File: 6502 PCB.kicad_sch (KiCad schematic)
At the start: 23 parts, among them J1 power_source, SW1 RESET, SW2 SW_Push, SW3 SW_Push, SW4 SW_Push, SW5 SW_Push, SW6 SW_Push, U1 W65C02S, U2 28C256, U3 62256, U4 W65C22, U5 74HC00, X1 1MHz

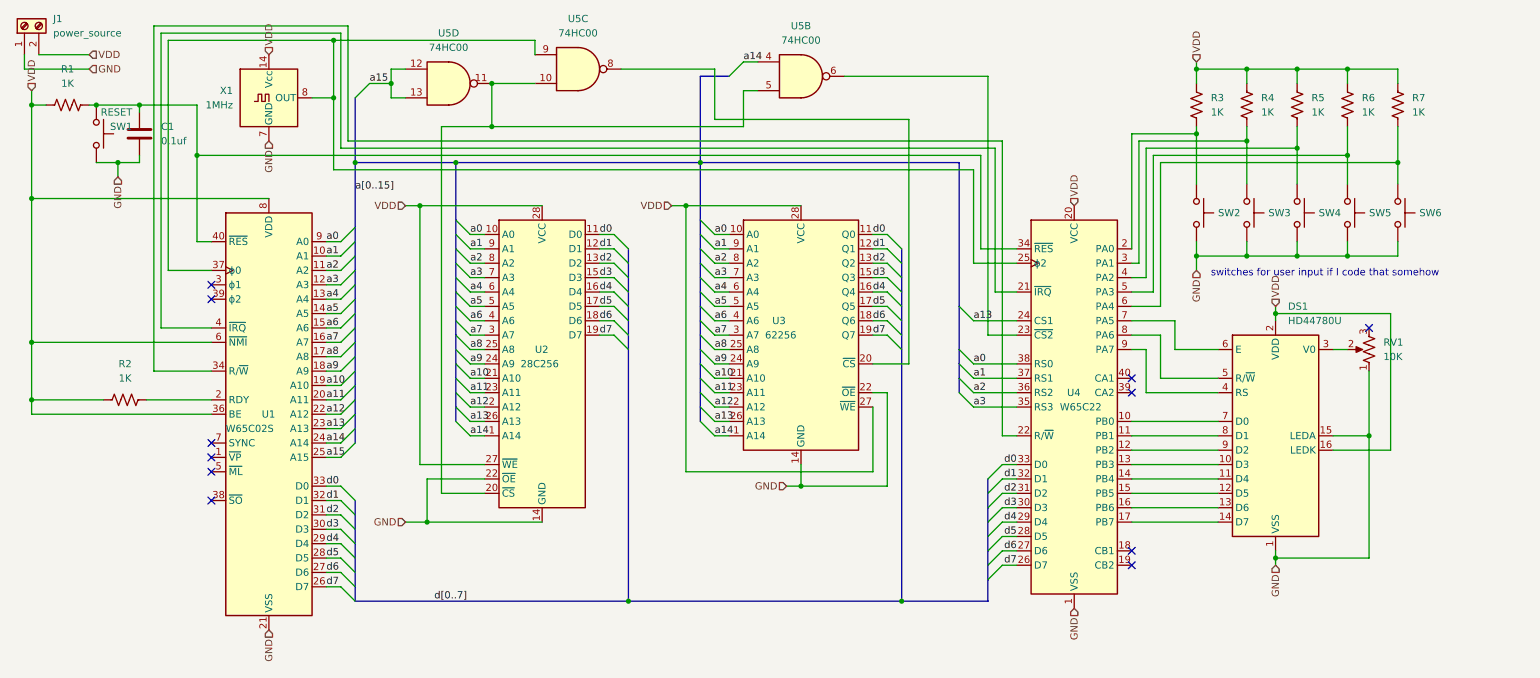
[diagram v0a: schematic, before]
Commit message: pretty much done
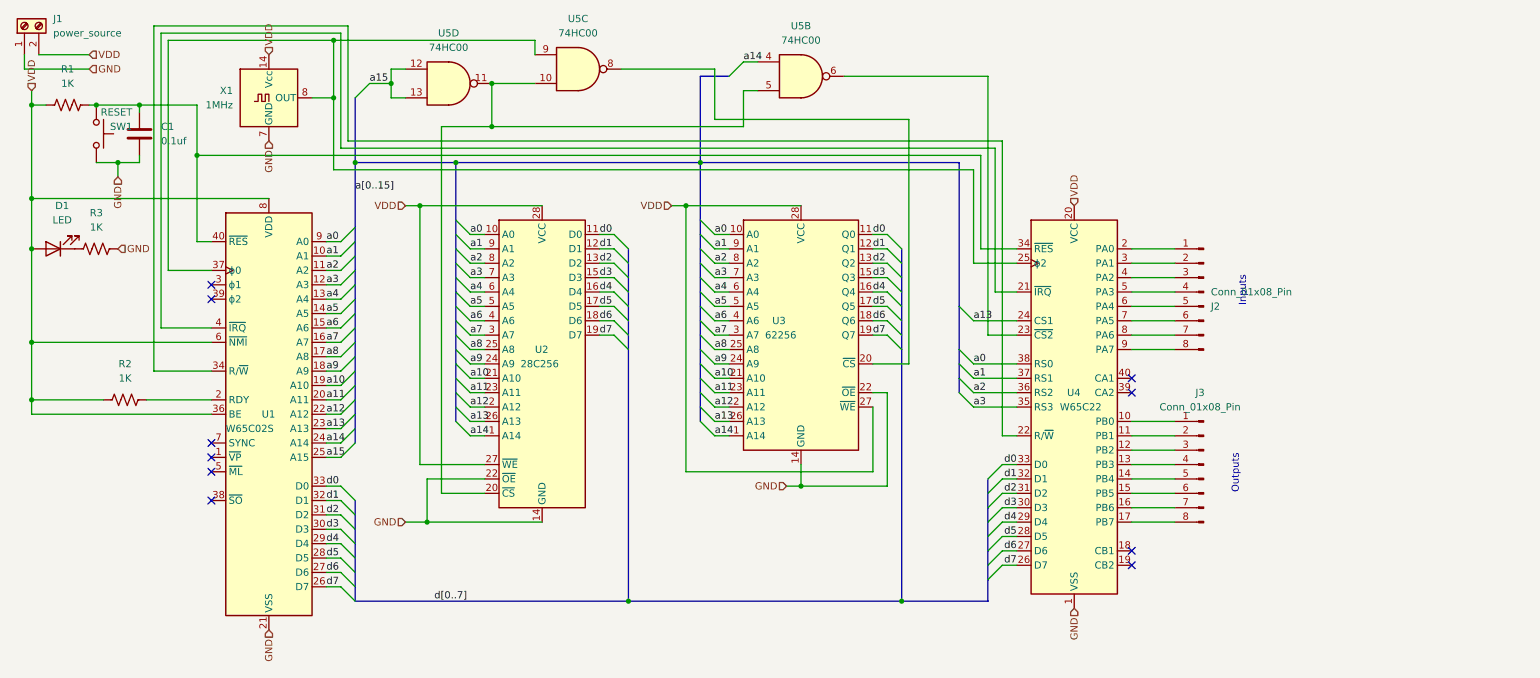
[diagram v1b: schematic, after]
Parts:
- removed DS1: HD44780U, Display:WC1602A, symbol HD44780U:HD44780U
- removed R4, R5, R6, R7: 1K, Resistor_SMD:R_0201_0603Metric_Pad0.64x0.40mm_HandSolder, symbol Device:R_US
- removed RV1: 10K, Potentiometer_SMD:Potentiometer_ACP_CA6-VSMD_Vertical, symbol Device:R_Potentiometer_US
- removed SW2, SW3, SW4, SW5, SW6: SW_Push, Button_Switch_SMD:SW_SPST_PTS645, symbol Switch:SW_Push
- added D1: LED, LED_SMD:LED_0201_0603Metric_Pad0.64x0.40mm_HandSolder, symbol Device:LED
- added J2, J3: Conn_01x08_Pin, Connector_PinHeader_1.00mm:PinHeader_1x08_P1.00mm_Vertical, symbol Connector:Conn_01x08_Pin
- C1: footprint Capacitor_SMD:CP_Elec_3x5.3 -> Capacitor_SMD:C_0201_0603Metric_Pad0.64x0.40mm_HandSolder
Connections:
- net GND: now also R3.2
- net VDD: now also D1.2 (A); no longer R3.2
- net at U4.4 (PA2): now also J2.3 (Pin_3)
- net at U4.3 (PA1): now also J2.2 (Pin_2)
- net at U4.13 (PB3): now also J3.4 (Pin_4)
- net at U4.14 (PB4): now also J3.5 (Pin_5)
- net at U4.15 (PB5): now also J3.6 (Pin_6)
- net at U4.16 (PB6): now also J3.7 (Pin_7)
- net at U4.17 (PB7): now also J3.8 (Pin_8)
- net at U4.9 (PA7): now also J2.8 (Pin_8)
- net at U4.8 (PA6): now also J2.7 (Pin_7)
- net at U4.7 (PA5): now also J2.6 (Pin_6)
- net at U4.10 (PB0): now also J3.1 (Pin_1)
- net at U4.11 (PB1): now also J3.2 (Pin_2)
- net at U4.12 (PB2): now also J3.3 (Pin_3)
- net at U4.2 (PA0): now also J2.1 (Pin_1); no longer R3.1
- net at U4.5 (PA3): now also J2.4 (Pin_4)
- net at U4.6 (PA4): now also J2.5 (Pin_5)
- new net: D1.1 (K), R3.1
- no-connect marks 11 -> 10
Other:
- note added: "Inputs"
- note added: "Outputs"
- note removed: "switches for user input if I code that somehow"

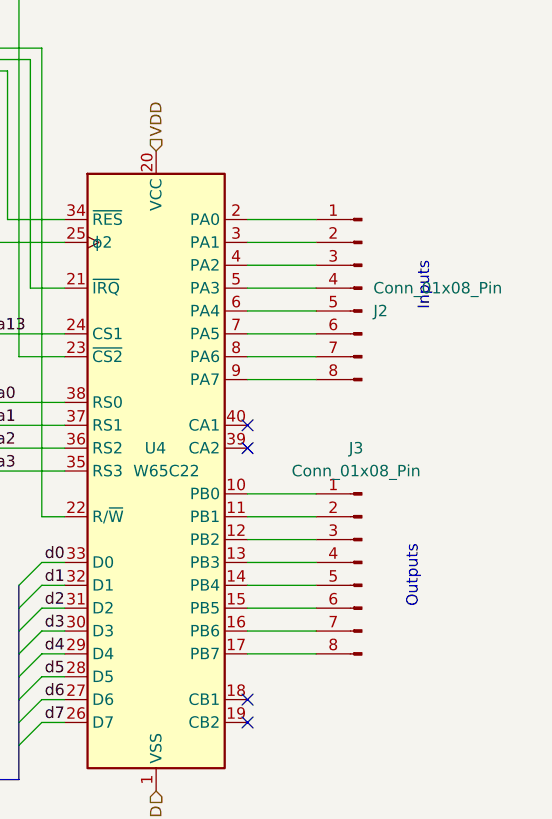
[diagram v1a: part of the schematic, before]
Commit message: Add files via upload
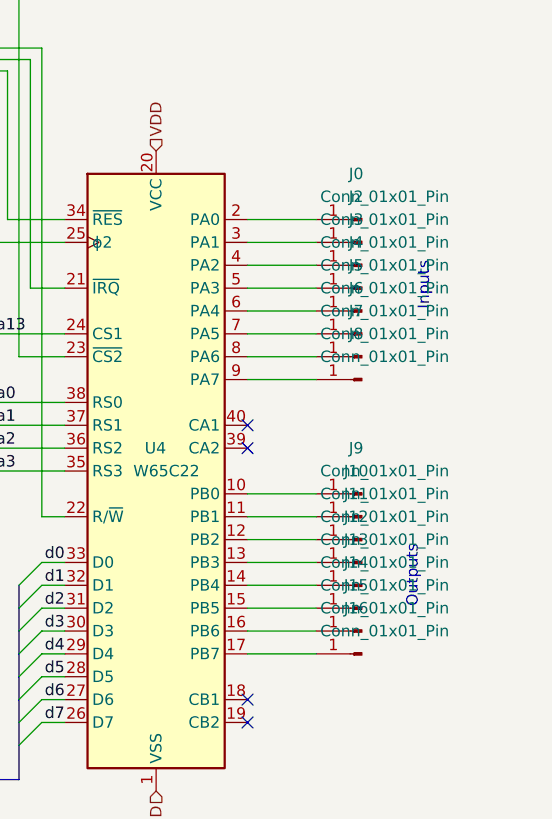
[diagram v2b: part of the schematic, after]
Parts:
- removed J2, J3: Conn_01x08_Pin, Connector_PinHeader_1.00mm:PinHeader_1x08_P1.00mm_Vertical, symbol Connector:Conn_01x08_Pin
- added J0, J10, J11, J12, J13, J14, J15, J16, J2, J3, J4, J5, J6, J7, J8, J9: Conn_01x01_Pin, Connector_PinHeader_1.00mm:PinHeader_1x01_P1.00mm_Vertical, symbol Connector:Conn_01x01_Pin
- C1: footprint Capacitor_SMD:C_0201_0603Metric_Pad0.64x0.40mm_HandSolder -> Capacitor_THT:C_Disc_D5.0mm_W2.5mm_P5.00mm
- D1: footprint LED_SMD:LED_0201_0603Metric_Pad0.64x0.40mm_HandSolder -> LED_THT:LED_D3.0mm
- R1, R2, R3: footprint Resistor_SMD:R_0201_0603Metric_Pad0.64x0.40mm_HandSolder -> Resistor_THT:R_Axial_DIN0204_L3.6mm_D1.6mm_P7.62mm_Horizontal
- SW1: footprint Button_Switch_SMD:SW_SPST_PTS645 -> Button_Switch_THT:SW_PUSH_6mm
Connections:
- net at U4.10 (PB0): now also J9.1 (Pin_1)
- net at U4.11 (PB1): now also J10.1 (Pin_1)
- net at U4.12 (PB2): now also J11.1 (Pin_1)
- net at U4.13 (PB3): now also J12.1 (Pin_1)
- net at U4.14 (PB4): now also J13.1 (Pin_1)
- net at U4.15 (PB5): now also J14.1 (Pin_1)
- net at U4.16 (PB6): now also J15.1 (Pin_1)
- net at U4.17 (PB7): now also J16.1 (Pin_1)
- net at U4.2 (PA0): now also J0.1 (Pin_1)
- net at U4.3 (PA1): now also J2.1 (Pin_1)
- net at U4.4 (PA2): now also J3.1 (Pin_1)
- net at U4.5 (PA3): now also J4.1 (Pin_1)
- net at U4.6 (PA4): now also J5.1 (Pin_1)
- net at U4.7 (PA5): now also J6.1 (Pin_1)
- net at U4.8 (PA6): now also J7.1 (Pin_1)
- net at U4.9 (PA7): now also J8.1 (Pin_1)

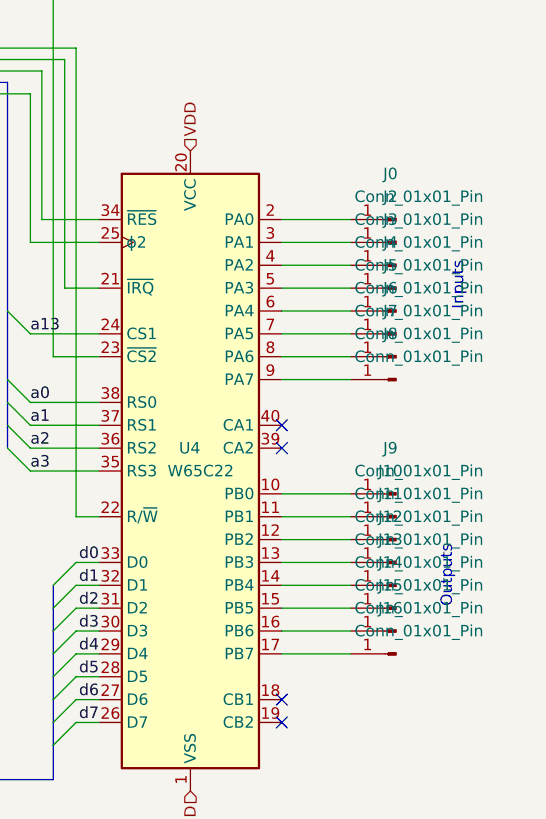
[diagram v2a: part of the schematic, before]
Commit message: pls work
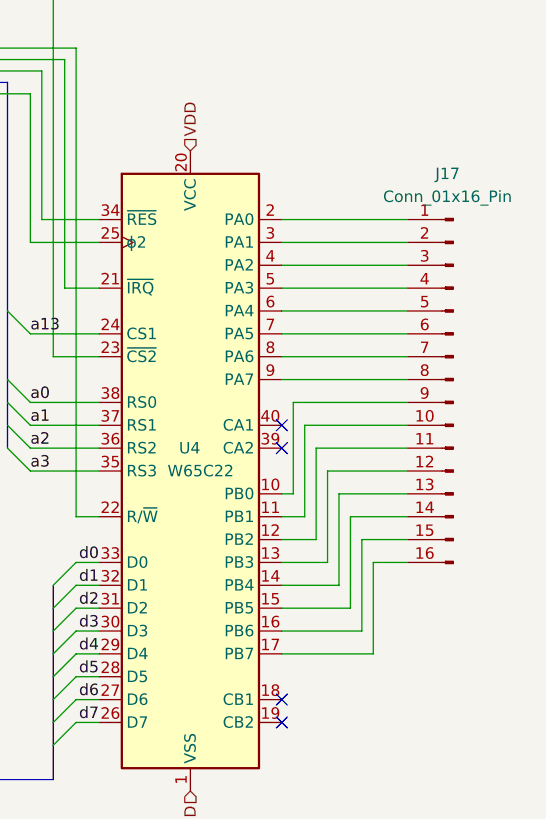
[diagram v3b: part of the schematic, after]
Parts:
- removed J0, J10, J11, J12, J13, J14, J15, J16, J2, J3, J4, J5, J6, J7, J8, J9: Conn_01x01_Pin, Connector_PinHeader_1.00mm:PinHeader_1x01_P1.00mm_Vertical, symbol Connector:Conn_01x01_Pin
- added J17: Conn_01x16_Pin, Connector_PinHeader_2.00mm:PinHeader_1x16_P2.00mm_Vertical, symbol Connector:Conn_01x16_Pin
- J1: footprint TerminalBlock:TerminalBlock_Altech_AK300-2_P5.00mm -> TerminalBlock:TerminalBlock_bornier-2_P5.08mm
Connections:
- net at U4.2 (PA0): now also J17.1 (Pin_1)
- net at U4.5 (PA3): now also J17.4 (Pin_4)
- net at U4.13 (PB3): now also J17.12 (Pin_12)
- net at U4.12 (PB2): now also J17.11 (Pin_11)
- net at U4.14 (PB4): now also J17.13 (Pin_13)
- net at U4.17 (PB7): now also J17.16 (Pin_16)
- net at U4.7 (PA5): now also J17.6 (Pin_6)
- net at U4.6 (PA4): now also J17.5 (Pin_5)
- net at U4.16 (PB6): now also J17.15 (Pin_15)
- net at U4.9 (PA7): now also J17.8 (Pin_8)
- net at U4.10 (PB0): now also J17.9 (Pin_9)
- net at U4.3 (PA1): now also J17.2 (Pin_2)
- net at U4.11 (PB1): now also J17.10 (Pin_10)
- net at U4.15 (PB5): now also J17.14 (Pin_14)
- net at U4.4 (PA2): now also J17.3 (Pin_3)
- net at U4.8 (PA6): now also J17.7 (Pin_7)
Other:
- note removed: "Inputs"
- note removed: "Outputs"
